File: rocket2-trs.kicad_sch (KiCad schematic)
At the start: 48 parts, among them J2 SMA, J3 ARM Cortex Debug, U4 AZ1117-3.3, U5 LoRA-E5, Y1 16MHz

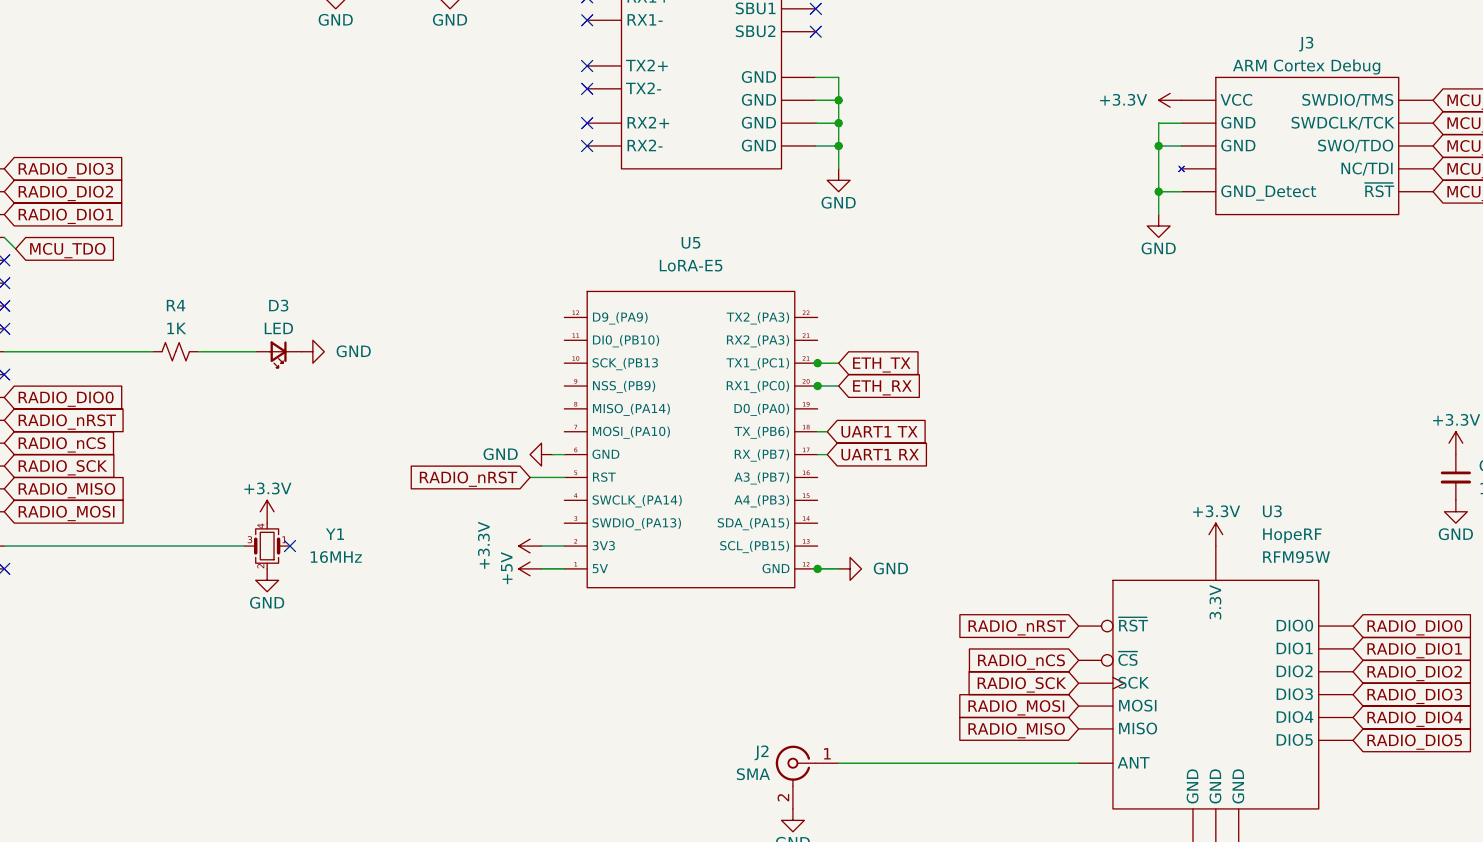
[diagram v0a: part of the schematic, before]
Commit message: TRS fixed
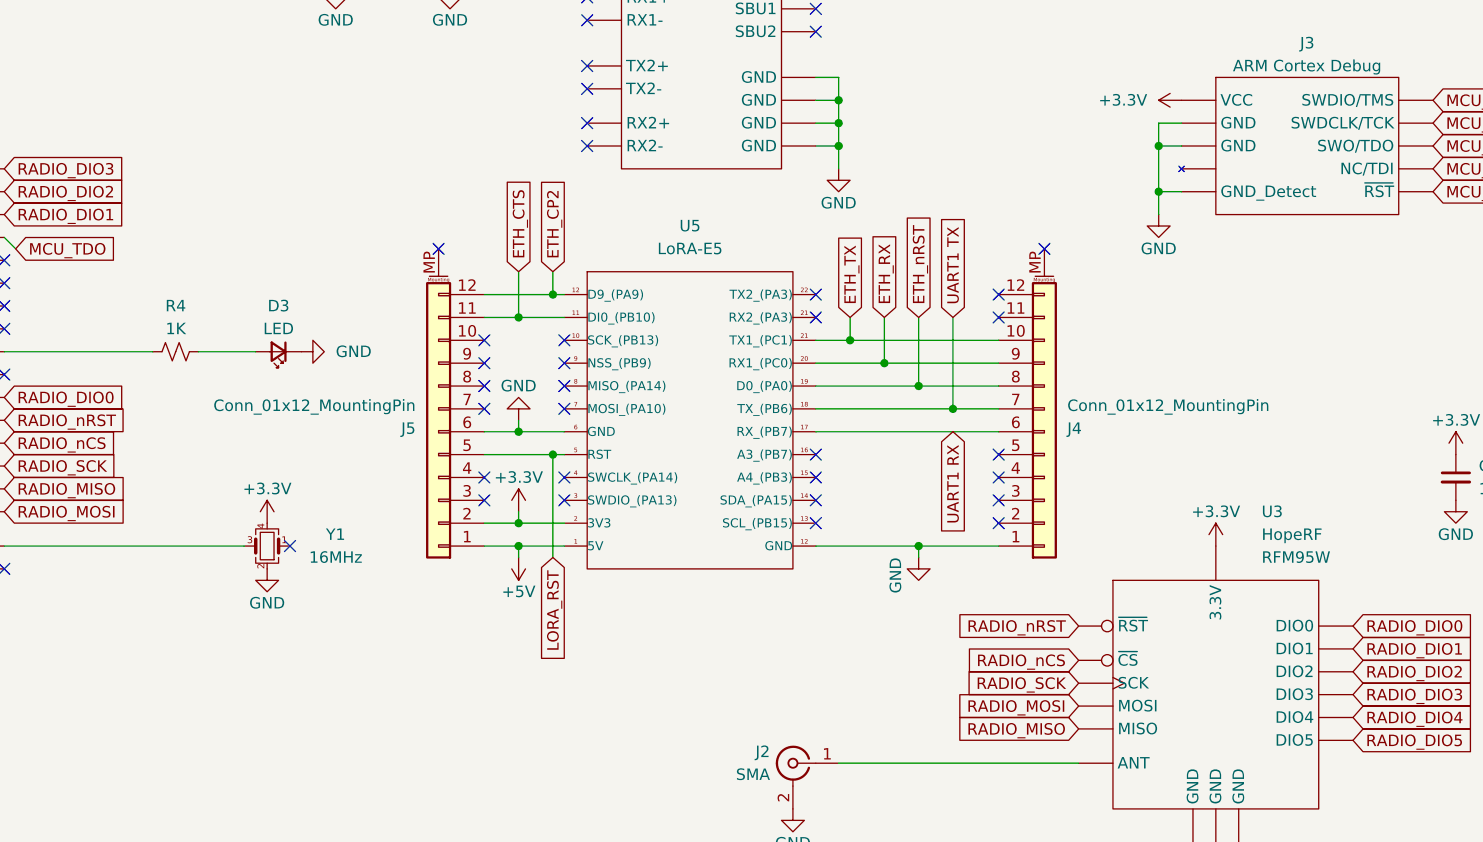
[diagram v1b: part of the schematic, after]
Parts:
- added J4, J5: Conn_01x12_MountingPin, symbol Connector_Generic_MountingPin:Conn_01x12_MountingPin
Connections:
- net +3.3V: now also J5.2 (Pin_2)
- net +5V: now also J5.1 (Pin_1)
- net ETH_CP2: now also U5.12 (GND), J5.12 (Pin_12)
- net ETH_CTS: now also U5.11 (DI0_(PB10)), J5.11 (Pin_11)
- net ETH_RX: now also J4.9 (Pin_9)
- net ETH_TX: now also J4.10 (Pin_10)
- net ETH_nRST: now also U5.19 (D0_(PA0)), J4.8 (Pin_8)
- net GND: now also J4.1 (Pin_1), J5.6 (Pin_6)
- net RADIO_nRST: no longer U5.5 (RST)
- net UART1 RX: now also J4.6 (Pin_6)
- net UART1 TX: now also J4.7 (Pin_7)
- new net LORA_RST: J5.5 (Pin_5), U5.5 (RST)
- no-connect marks 21 -> 47
